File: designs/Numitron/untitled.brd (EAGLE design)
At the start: 40 x 86 mm, 10 parts, among them IC2 TLC5916IN, IC3 TLC5916IN, IC4 TLC5916IN, IC5 TLC5916IN

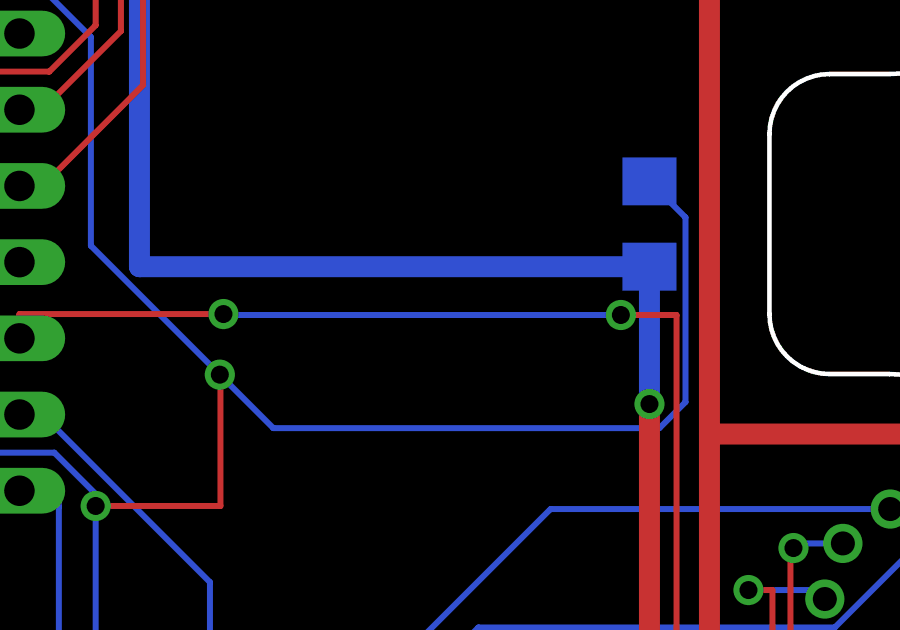
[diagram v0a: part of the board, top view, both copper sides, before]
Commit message: added last design tunes
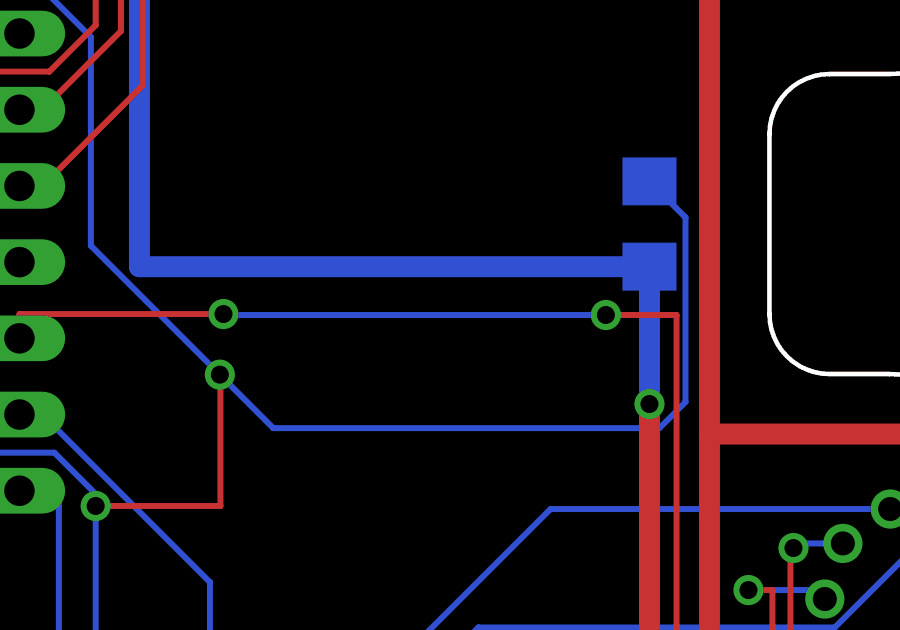
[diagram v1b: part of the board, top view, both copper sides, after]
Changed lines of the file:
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@@
 <?xml version="1.0" encoding="utf-8"?>
 <!DOCTYPE eagle SYSTEM "eagle.dtd">
-<eagle version="9.4.2">
+<eagle version="9.5.1">
 <drawing>
 <settings>
-<setting alwaysvectorfont="yes"/>
+<setting alwaysvectorfont="no"/>
 <setting verticaltext="up"/>
 </settings>
@@
 <wire x1="18.246459375" y1="18.3272" x2="10.61405" y2="18.3272" width="0.2" layer="1"/>
 <wire x1="10.61405" y1="18.3272" x2="9.08" y2="16.79315" width="0.2" layer="1"/>
-<via x="24.0468" y="39.967953125" extent="1-16" drill="0.6"/>
-<wire x1="24.0468" y1="39.967953125" x2="10.8" y2="39.967953125" width="0.2" layer="16"/>
+<via x="23.5468" y="39.967953125" extent="1-16" drill="0.6"/>
+<wire x1="23.5468" y1="39.967953125" x2="10.8" y2="39.967953125" width="0.2" layer="16"/>
 <via x="10.8" y="40" extent="1-16" drill="0.6"/>
 <wire x1="10.8" y1="40" x2="4" y2="40" width="0.2" layer="1"/>
 <wire x1="4" y1="40" x2="4" y2="39.19" width="0.2" layer="1"/>
 <wire x1="10.8" y1="39.967953125" x2="10.8" y2="40" width="0.2" layer="16"/>
-<wire x1="25.903203125" y1="39.967953125" x2="24.0468" y2="39.967953125" width="0.2" layer="1"/>
+<wire x1="25.903203125" y1="39.967953125" x2="23.5468" y2="39.967953125" width="0.2" layer="1"/>
 <wire x1="25.903203125" y1="25.98394375" x2="25.903203125" y2="39.967953125" width="0.2" layer="1"/>
 </signal>
